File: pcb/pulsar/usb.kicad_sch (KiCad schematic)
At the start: 6 parts, among them J1 USB_C_Receptacle, U1 PRTR5V0U2X

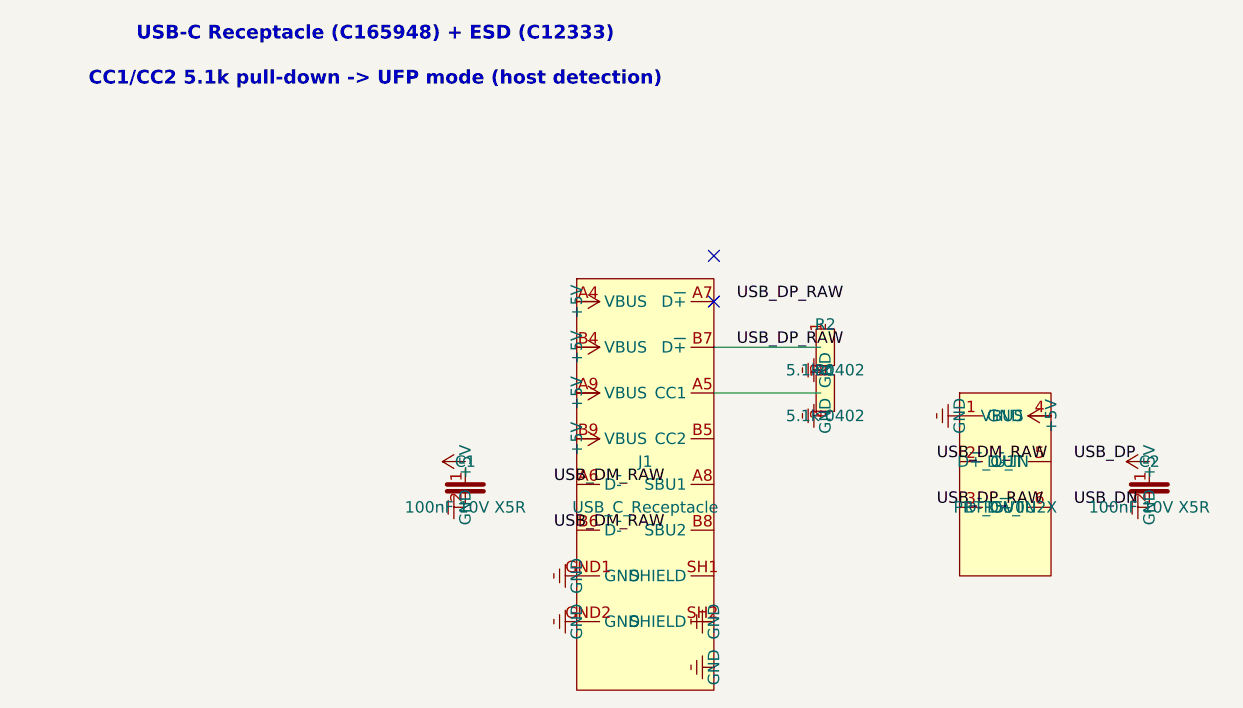
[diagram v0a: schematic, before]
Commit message: feat: let everything to route
Signed-off-by: Axel Ibarrondo <135344010+Axel84727@users.noreply.github.com>
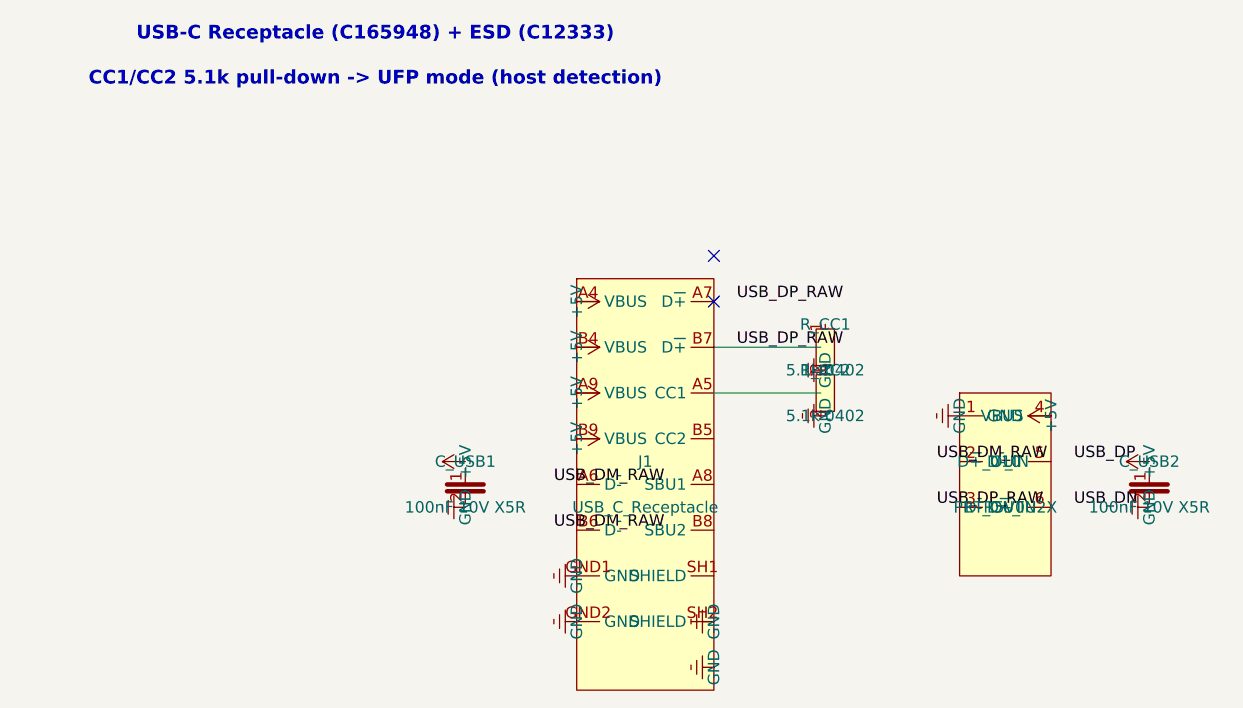
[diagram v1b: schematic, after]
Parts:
- renumbered C1 to C_USB1, C2 to C_USB2, R2 to R_CC1, R1 to R_CC2, U1 to U10
